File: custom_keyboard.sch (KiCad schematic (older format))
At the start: 84 parts

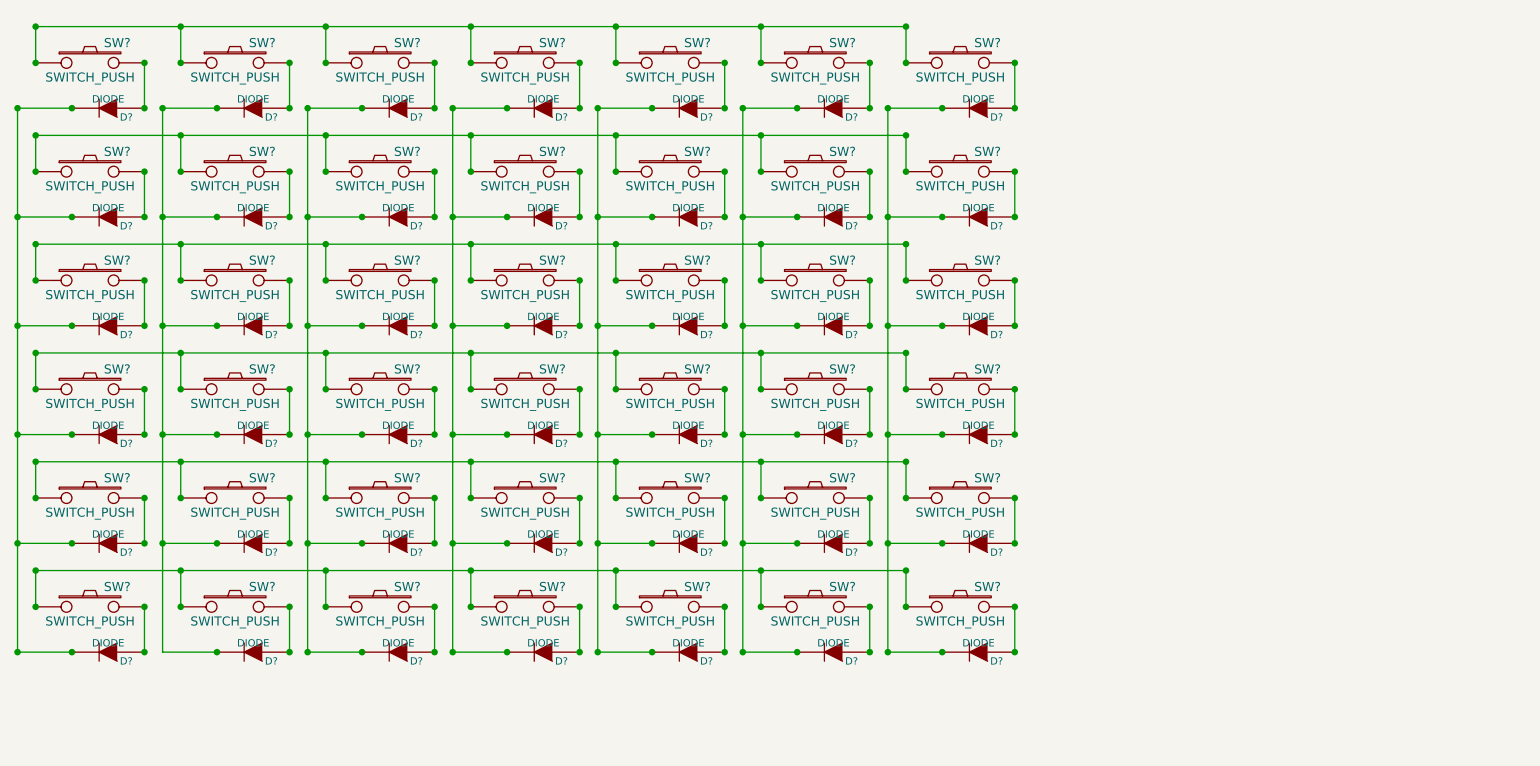
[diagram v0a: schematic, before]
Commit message: asdfasd
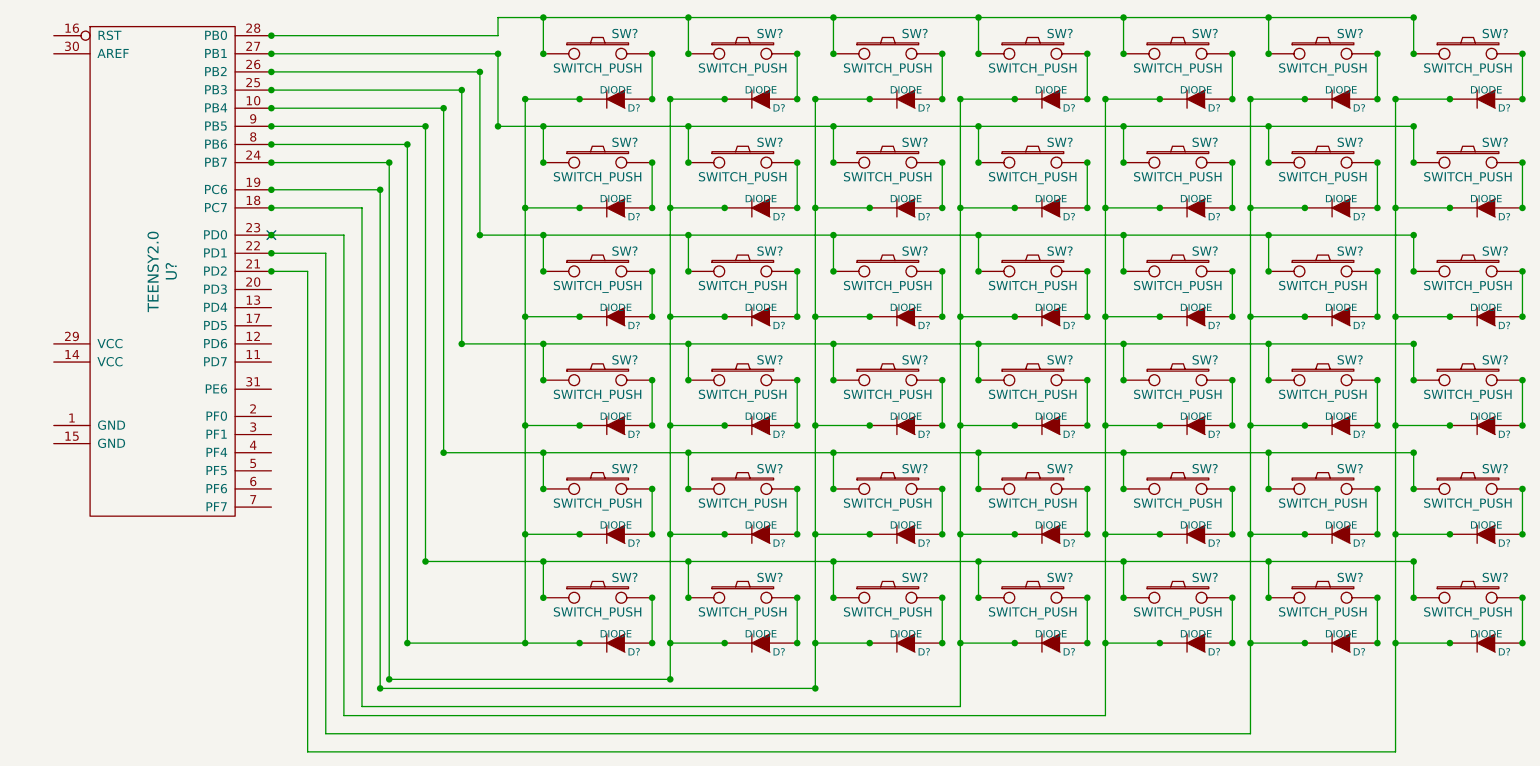
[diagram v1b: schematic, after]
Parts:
- added U?: TEENSY2.0, symbol TEENSY2.0
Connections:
- net at SW?.1, SW?.1, SW?.1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: now also U?.28 (PB0)
- net at D?.2 (K), D?.2 (K), D?.2 (K)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: now also U?.8 (PB6)
- net at SW?.1, SW?.1, SW?.1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: now also U?.27 (PB1)
- net at SW?.1, SW?.1, SW?.1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: now also U?.26 (PB2)
- net at SW?.1, SW?.1, SW?.1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: now also U?.25 (PB3)
- net at SW?.1, SW?.1, SW?.1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: now also U?.10 (PB4)
- net at SW?.1, SW?.1, SW?.1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: now also U?.9 (PB5)
- net at D?.2 (K), D?.2 (K), D?.2 (K)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: now also U?.24 (PB7)
- net at D?.2 (K), D?.2 (K), D?.2 (K)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: now also U?.19 (PC6)
- net at D?.2 (K), D?.2 (K), D?.2 (K)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: now also U?.18 (PC7)
- net at D?.2 (K), D?.2 (K), D?.2 (K)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: now also U?.23 (PD0)
- net at D?.2 (K), D?.2 (K), D?.2 (K)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: now also U?.22 (PD1)
- net at D?.2 (K), D?.2 (K), D?.2 (K)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: now also U?.21 (PD2)
- no-connect marks 0 -> 1
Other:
- moved on the sheet: D?, SW?
